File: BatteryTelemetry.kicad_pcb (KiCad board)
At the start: 2 copper layers, 137 parts, among them IC1 BQ76925PWR, IC2 BQ76925PWR, IC3 BQ76925PWR, IC4 BQ76925PWR, J1 Conn_01x07_Pin, J2 Conn_01x07_Pin, J3 Conn_01x07_Pin, J4 Conn_01x07_Pin, J5 USB_C_Receptacle_USB2.0, J6 Conn_01x04_Socket, J7 Conn_01x03_Socket, J8 Conn_01x03_Socket, Q1 ZXTP25040DFHTA, SW1 SW_Push, SW2 SW_Push, SW3 SW_SPDT, U1 RP2040, U2 NCP1117-3.3_SOT223, U3 W25Q128JVS, U4 TCA9548APWR, Y1 ABM10AIG-12.000MHZ-4Z-T3

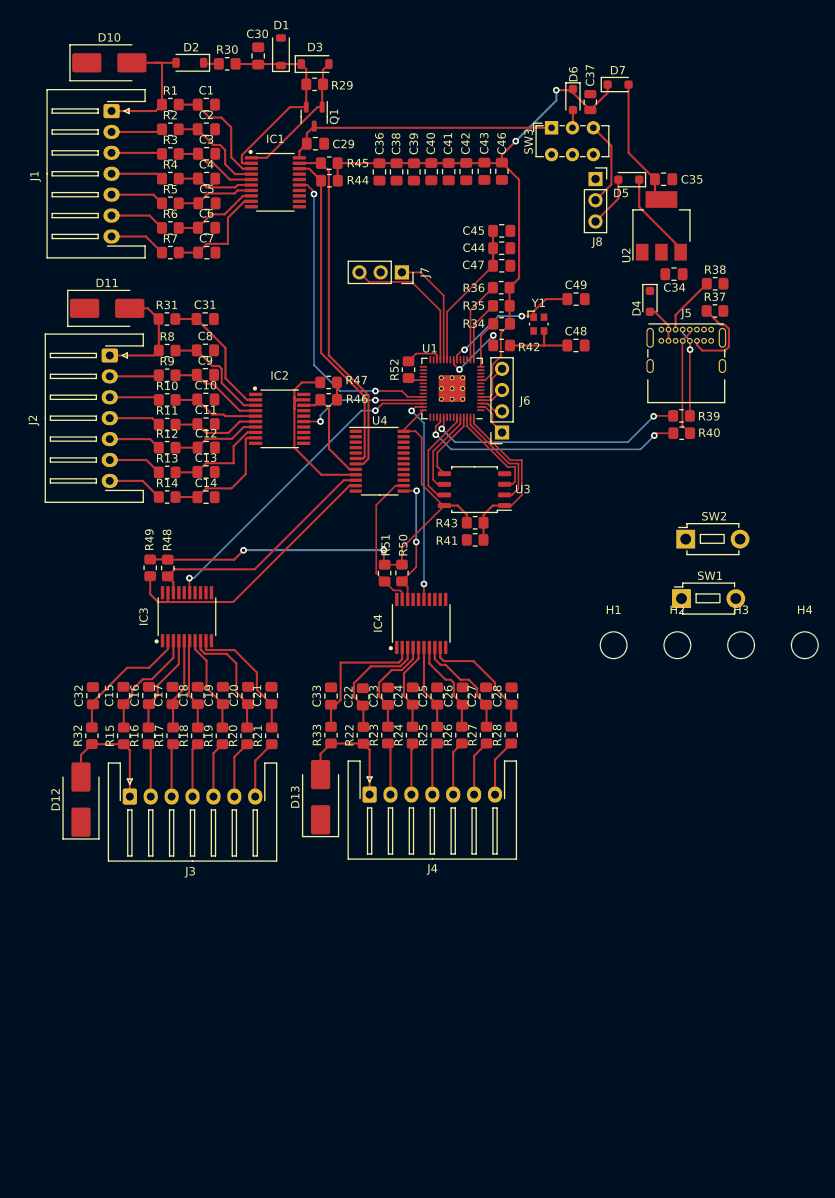
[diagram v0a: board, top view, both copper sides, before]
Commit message: Layout Complete
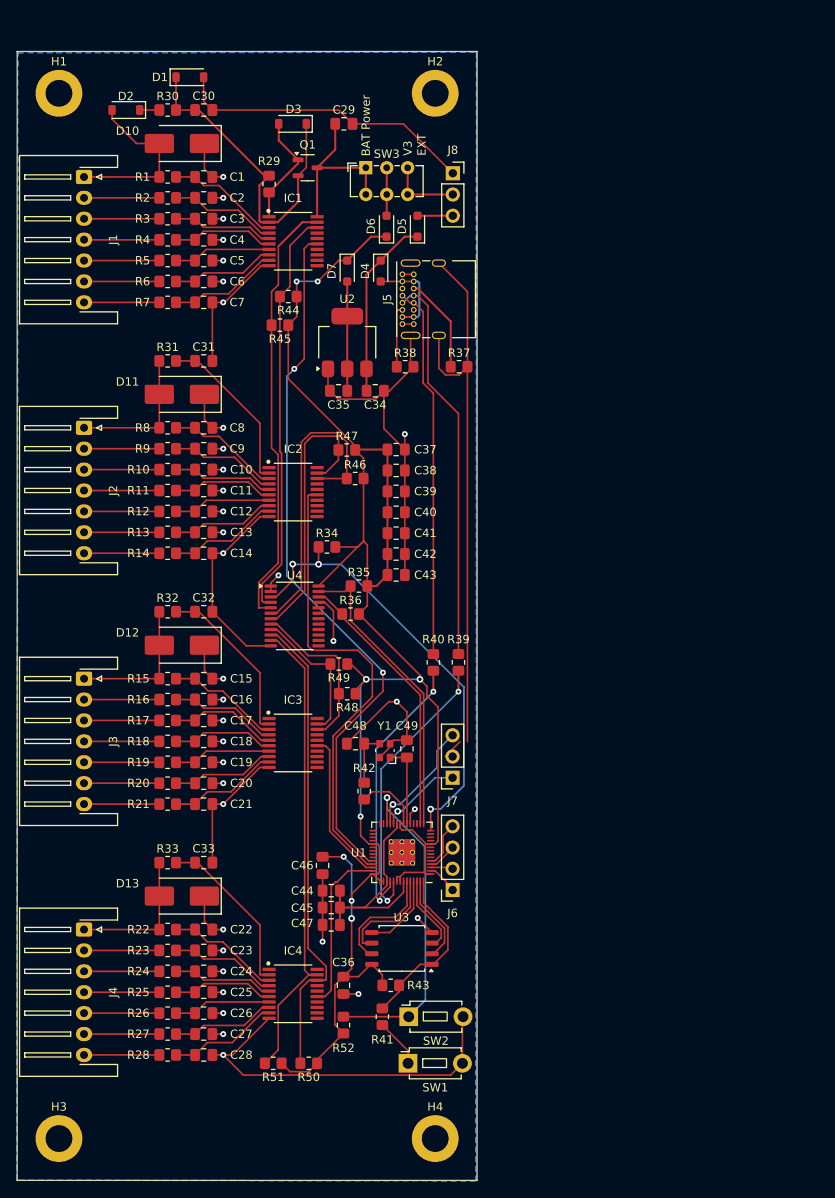
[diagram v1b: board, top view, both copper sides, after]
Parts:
- C37: footprint Capacitor_SMD:C_0805_2012Metric -> Capacitor_SMD:C_0805_2012Metric_Pad1.18x1.45mm_HandSolder
- H1, H2, H3, H4: footprint MountingHole:MountingHole_3.2mm_M3 -> MountingHole:MountingHole_3.2mm_M3_DIN965_Pad
- moved H3 100.7 mm to (30.0, 155.0)
- moved C36 97.4 mm to (64.0, 136.7)
- moved H1 93.6 mm to (30.0, 30.0)
- moved C46 85.7 mm to (61.5, 122.3)
- moved C45 83.5 mm to (62.6, 127.4), turned to 180 degrees
- moved C47 81.4 mm to (62.6, 129.4), turned to 180 degrees
- moved C44 79.5 mm to (62.6, 125.3), turned to 180 degrees
- moved R52 78.8 mm to (64.0, 141.4)
- moved H4 73.7 mm to (75.0, 155.0)
- moved H2 72.1 mm to (75.0, 30.0)
- moved SW2 66.0 mm to (71.8, 140.4)
- moved SW1 64.5 mm to (71.8, 146.0)
- moved J7 60.7 mm to (77.1, 111.8), turned to 180 degrees
- moved R51 60.1 mm to (55.6, 146.0), turned to 180 degrees
- moved R50 59.7 mm to (59.9, 146.0), turned to 180 degrees
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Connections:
- SW3 pad 4: (no net) -> /V3_BAT
- SW3 pad 5: (no net) -> Net-(D6-A)
- SW3 pad 6: (no net) -> /V3_EXT
- U4 pad 10: /SDA_BAT3 -> /SDA_BAT4
- U4 pad 11: /SCL_BAT3 -> /SCL_BAT4
- U4 pad 13: /SDA_BAT4 -> unconnected-(U4-SD4-Pad13)
- U4 pad 14: /SCL_BAT4 -> unconnected-(U4-SC4-Pad14)
- U4 pad 4: unconnected-(U4-SD0-Pad4) -> /SDA_BAT1
- U4 pad 5: unconnected-(U4-SC0-Pad5) -> /SCL_BAT1
- U4 pad 6: /SDA_BAT1 -> /SDA_BAT2
- U4 pad 7: /SCL_BAT1 -> /SCL_BAT2
- U4 pad 8: /SDA_BAT2 -> /SDA_BAT3
- U4 pad 9: /SCL_BAT2 -> /SCL_BAT3
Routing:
- net GND: track 0.00 -> 353.9 mm, vias 0 -> 36
- net +3V3: track 136.7 -> 222.7 mm, vias 4 -> 8
- net /RESET: track 5.75 -> 53.6 mm, vias 0 -> 3
- net /BAT1: track 37.5 -> 85.0 mm
- net /SDA_BAT4: track 15.6 -> 56.8 mm, vias 2 -> 0
- net /BAT2: track 15.8 -> 55.9 mm, vias 2 -> 0
- net /SCL_BAT4: track 18.0 -> 57.0 mm
- net /RUN: track 4.41 -> 39.9 mm, vias 0 -> 1
- net /USB_D+: track 11.8 -> 47.1 mm, vias 1 -> 0
- net /USB_D-: track 13.1 -> 44.7 mm
- net /I2C0 SDA: track 7.40 -> 36.1 mm
- net /SDA_BAT2: track 12.8 -> 37.4 mm
- net /I2C0 SCL: track 9.73 -> 32.6 mm
- net /BAT3: track 38.4 -> 18.4 mm, vias 2 -> 0
- net /SCL_BAT3: track 35.1 -> 17.2 mm
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- added copper zone on B.Cu, net GND
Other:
- board outline added: 55 x 135 mm
- board text added: "BAT Power"
- board text added: "CTS"
- board text added: "EXT"
- board text added: "GND"
- board text added: "Input Power"
- board text added: "RTS"
- board text added: "RX"
- board text added: "SWCLK"
- board text added: "SWD"
- board text added: "SWD Debug Breakout"
- board text added: "TX"
- board text added: "UART Breakout"
- board text added: "V3"
- board text added: "V5 (or)"
